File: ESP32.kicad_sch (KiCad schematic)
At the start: 35 parts, among them J4 JTAG, Q1 MMBT3904, Q2 MMBT3904, U1 ESP-WROVER-32, U3 CH340G, Y1 12M

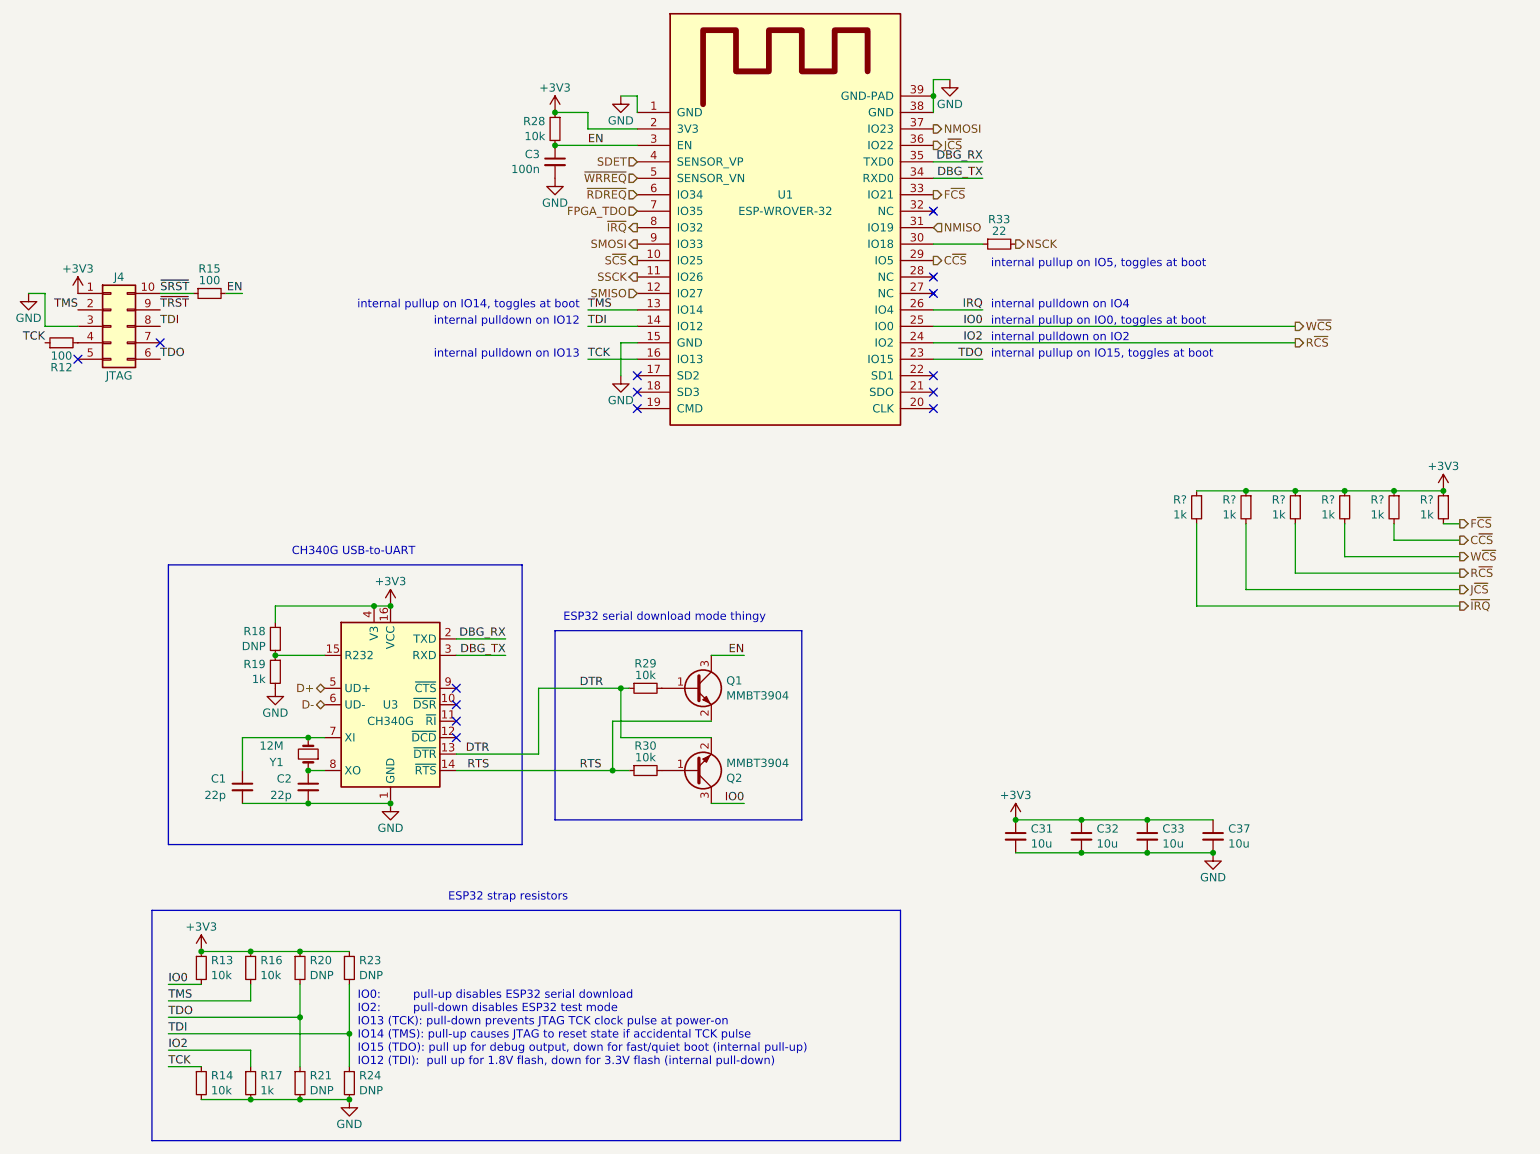
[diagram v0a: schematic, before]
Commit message: Revert "work on FPGA"
This reverts commit a96523e8d17974c7c48efc8a38ae046f7948cd49.
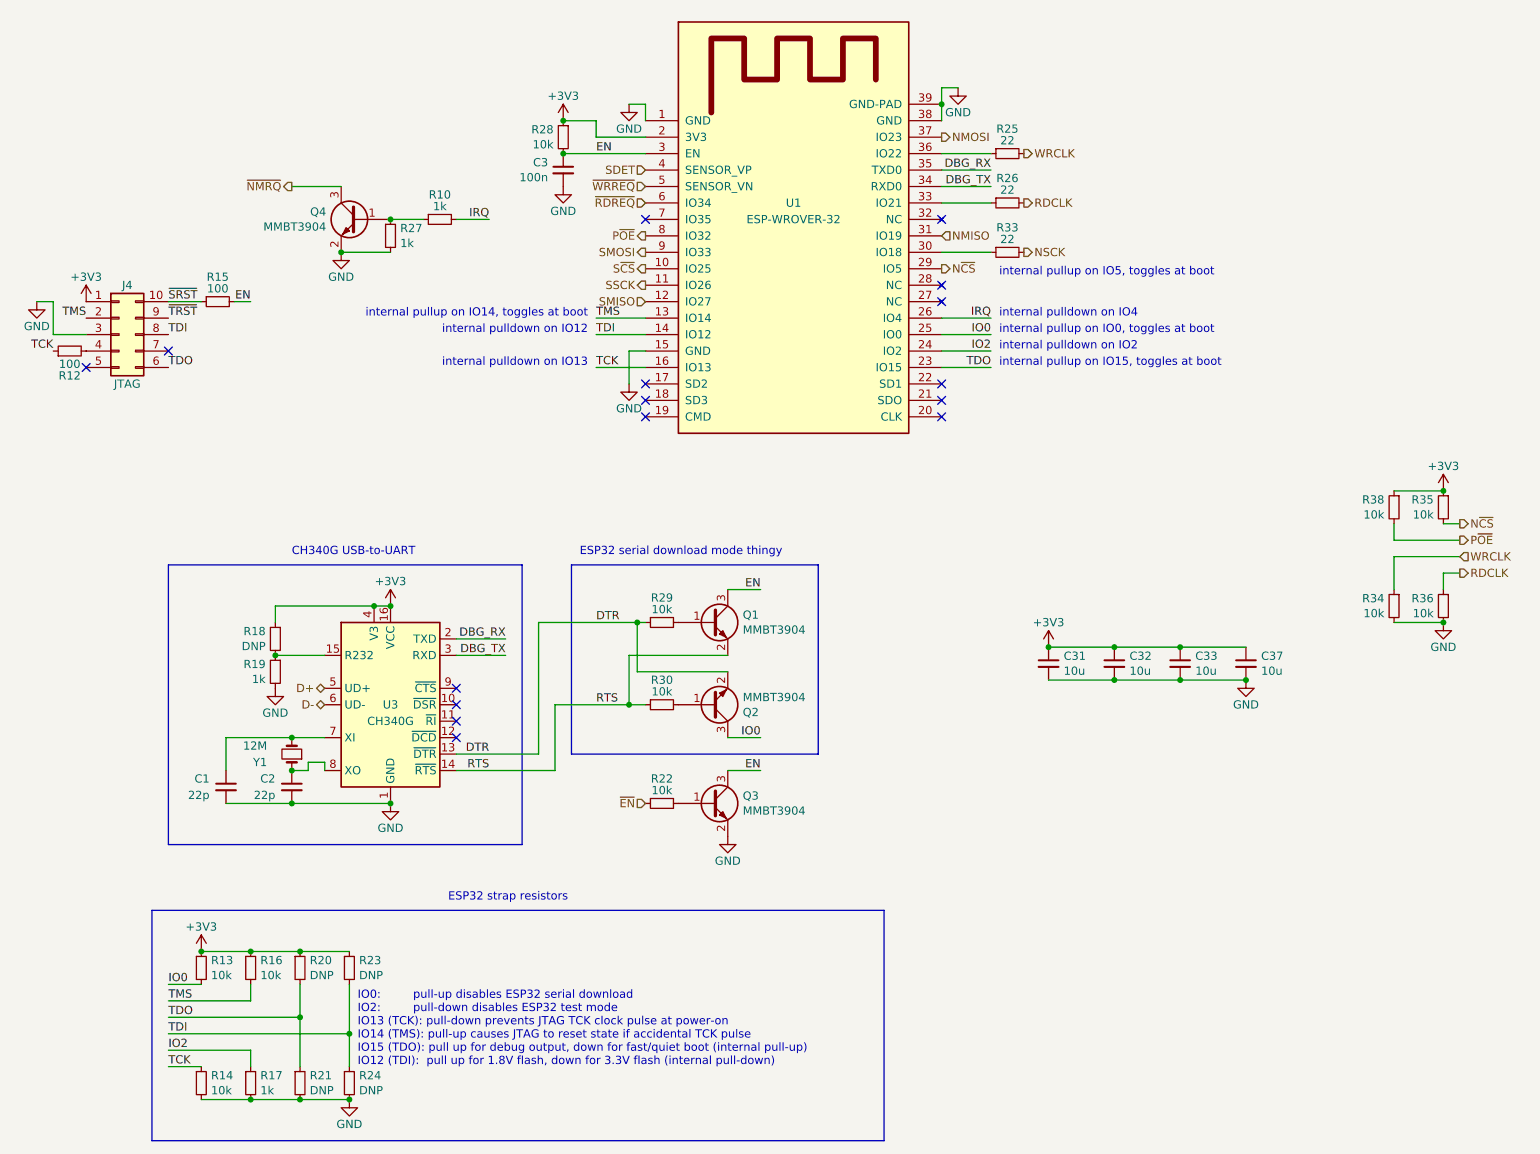
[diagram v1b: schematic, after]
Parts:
- removed R? (x6): 1k, stdpads:R_0805, symbol Device:R_Small
- added Q3, Q4: MMBT3904, stdpads:SOT-23, symbol Transistor_BJT:MMBT3904
- added R10, R27: 1k, stdpads:R_0805, symbol Device:R_Small
- added R22, R34, R35, R36, R38: 10k, stdpads:R_0805, symbol Device:R_Small
- added R25, R26: 22, stdpads:R_0805, symbol Device:R_Small
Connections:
- net +3V3: now also R35.1, R38.1
- net EN: now also Q3.3 (C)
- net GND: now also Q3.2 (E), Q4.2 (E), R27.2, R34.2, R36.2
- net IRQ: now also R10.2
- net C~{CS} renamed N~{CS}
- net N~{CS}: now also R35.2
- net FPGA_TDO: no longer names the net of U1.7 (IO35)
- net F~{CS}: no longer names the net of U1.33 (IO21)
- net F~{CS}: now also R26.1
- net J~{CS}: no longer names the net of U1.36 (IO22)
- net J~{CS}: now also R25.1
- net R~{CS} renamed IO2
- net W~{CS} renamed IO0
- net ~{IRQ} renamed P~{OE}
- net P~{OE}: now also R38.2
- new net: Q4.1 (B), R10.1, R27.1
- new net: Q3.1 (B), R22.2
- new net RDCLK: R26.2, R36.1
- new net WRCLK: R25.2, R34.1
- new net ~{EN}: R22.1
- new net ~{NMRQ}: Q4.3 (C)
- no-connect marks 15 -> 16
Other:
- moved on the sheet: C1, C2, C3, C31, C32, C33, C37, J4, Q1, Q2, R12, R15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

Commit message: work on FPGA
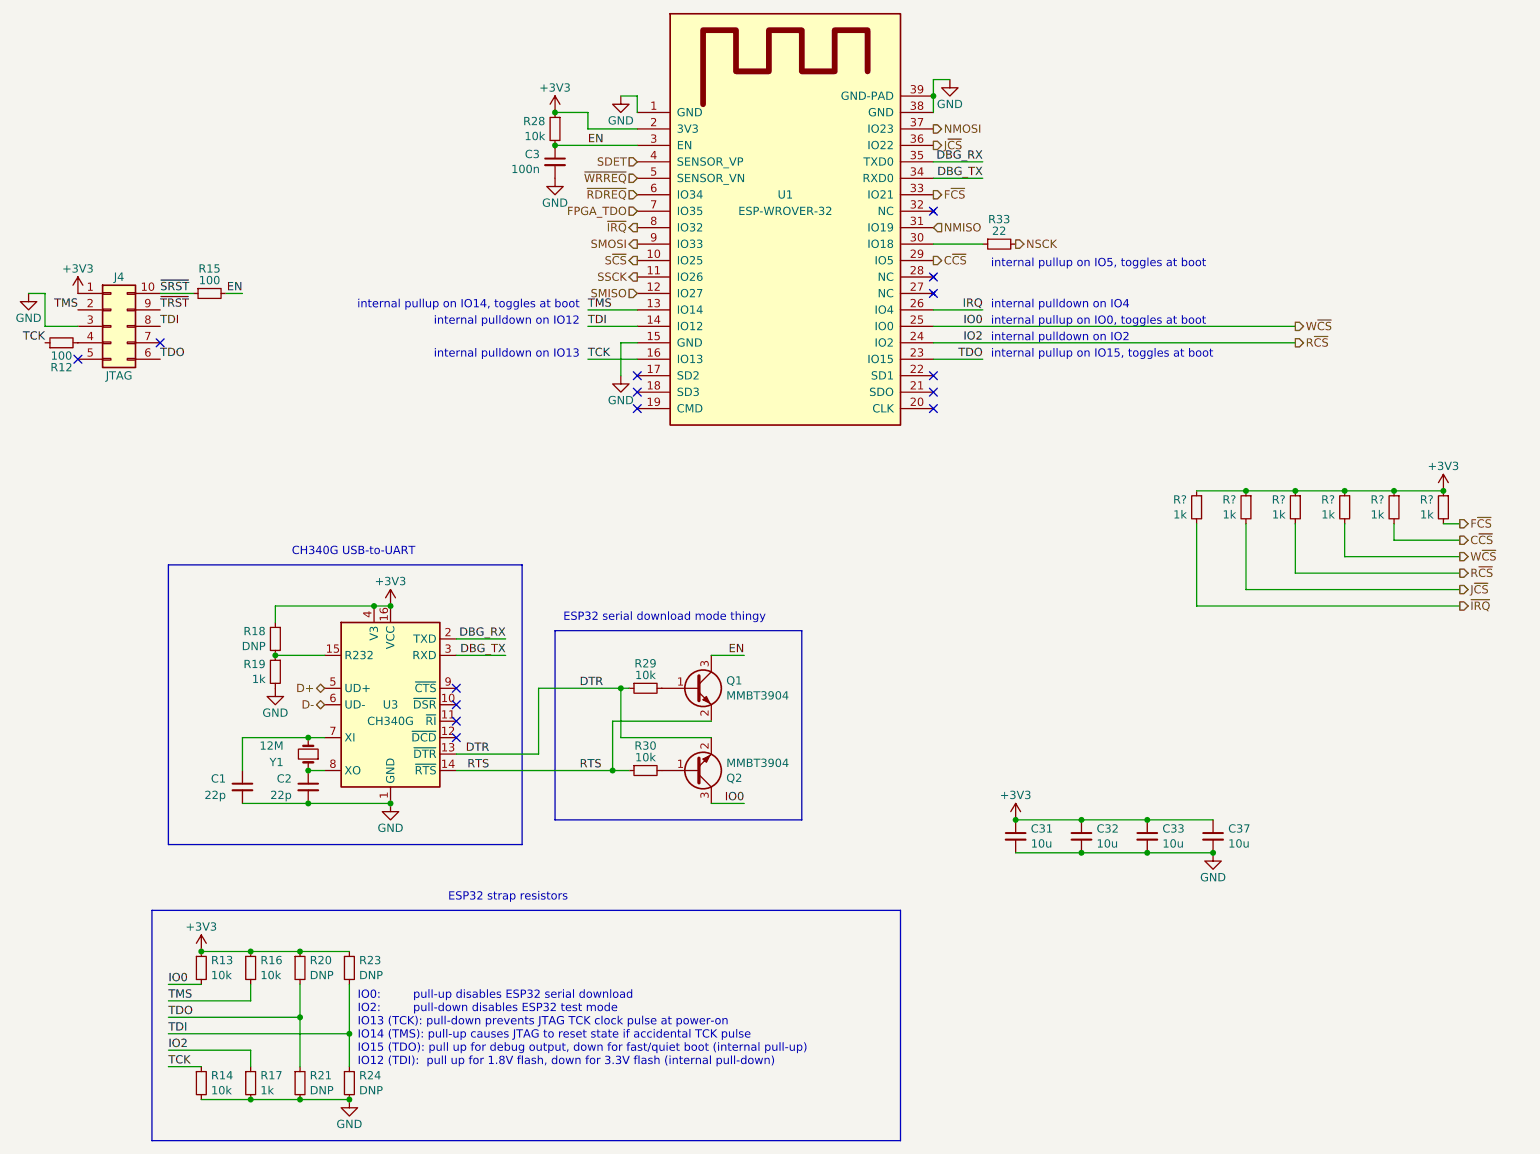
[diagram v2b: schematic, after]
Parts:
- removed Q3, Q4: MMBT3904, stdpads:SOT-23, symbol Transistor_BJT:MMBT3904
- removed R10, R27: 1k, stdpads:R_0805, symbol Device:R_Small
- removed R22, R34, R35, R36, R38: 10k, stdpads:R_0805, symbol Device:R_Small
- removed R25, R26: 22, stdpads:R_0805, symbol Device:R_Small
- added R? (x6): 1k, stdpads:R_0805, symbol Device:R_Small
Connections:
- net +3V3: now also R?.1, R?.1, R?.1, R?.1, R?.1, R?.1
- net F~{CS}: now reaches U1.33 (IO21)
- net F~{CS}: now also R?.2
- net J~{CS}: now reaches U1.36 (IO22)
- net J~{CS}: now also R?.2
- net FPGA_TDO: now reaches U1.7 (IO35)
- net IO0 renamed W~{CS}
- net W~{CS}: now also R?.2
- net IO2 renamed R~{CS}
- net R~{CS}: now also R?.2
- net N~{CS} renamed C~{CS}
- net C~{CS}: now also R?.2
- net P~{OE} renamed ~{IRQ}
- net ~{IRQ}: now also R?.2
- no-connect marks 16 -> 15
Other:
- moved on the sheet: C1, C2, C3, C31, C32, C33, C37, J4, Q1, Q2, R12, R15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
